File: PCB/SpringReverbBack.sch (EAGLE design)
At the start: 39 parts, among them IC4_DRV_RCVR TL072

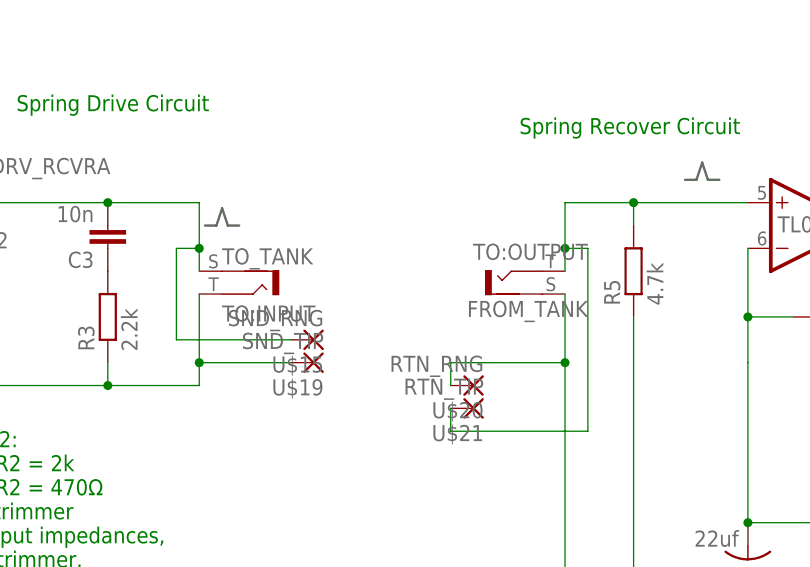
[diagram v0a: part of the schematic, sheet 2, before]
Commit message: Updated to Eagle 7.2
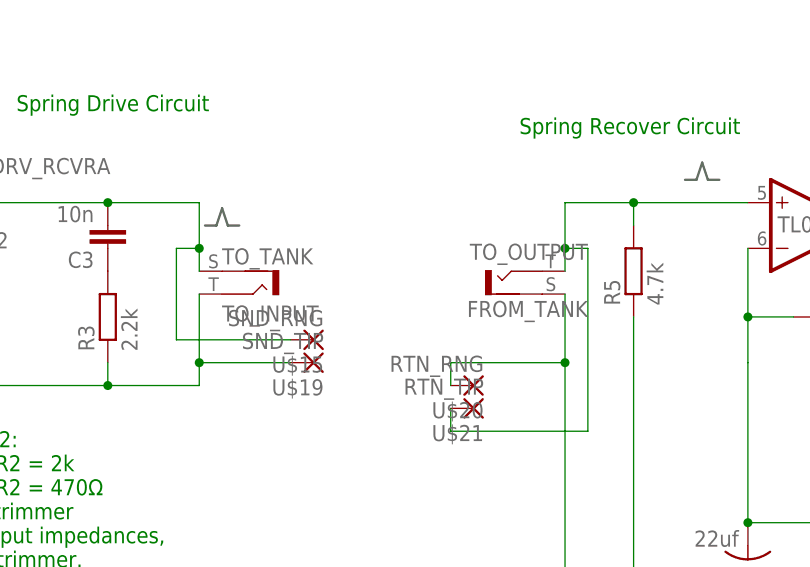
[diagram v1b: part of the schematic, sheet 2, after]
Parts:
- renumbered TO:INPUT to TO_INPUT, TO:OUTPUT to TO_OUTPUT
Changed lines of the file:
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@@
 <?xml version="1.0" encoding="utf-8"?>
 <!DOCTYPE eagle SYSTEM "eagle.dtd">
-<eagle version="6.4">
+<eagle version="7.2.0">
 <drawing>
 <settings>
@@
 <part name="C2" library="SparkFun-Passives" deviceset="CAP_POL" device="PTH2" value="10uf"/>
 <part name="SUPPLY4" library="supply2" deviceset="GND" device=""/>
-<part name="TO:INPUT" library="con-lumberg" deviceset="BTOR1" device="" value="TO_TANK"/>
+<part name="TO_INPUT" library="con-lumberg" deviceset="BTOR1" device="" value="TO_TANK"/>
 <part name="R3" library="TomW" deviceset="R-EU_" device="STANDARD_RESISTOR" value="2.2k"/>
 <part name="C3" library="TomW" deviceset="C-EU" device="050-024X044" value="10n"/>
-<part name="TO:OUTPUT" library="con-lumberg" deviceset="BTOR1" device="" value="FROM_TANK"/>
+<part name="TO_OUTPUT" library="con-lumberg" deviceset="BTOR1" device="" value="FROM_TANK"/>
 <part name="R4" library="TomW" deviceset="R-EU_" device="STANDARD_RESISTOR" value="22R"/>
 <part name="C8" library="SparkFun-Passives" deviceset="CAP_POL" device="PTH2" value="22uf"/>
@@
 <instance part="C2" gate="G$1" x="33.02" y="71.12"/>
 <instance part="SUPPLY4" gate="GND" x="38.1" y="43.18"/>
-<instance part="TO:INPUT" gate="G$1" x="81.28" y="88.9" rot="MR180"/>
+<instance part="TO_INPUT" gate="G$1" x="81.28" y="88.9" rot="MR180"/>
 <instance part="R3" gate="G$1" x="68.58" y="86.36" rot="R90"/>
 <instance part="C3" gate="G$1" x="68.58" y="93.98" rot="R180"/>
@@
 <attribute name="VALUE" x="143.002" y="95.758" size="1.778" layer="96"/>
 </instance>
-<instance part="TO:OUTPUT" gate="G$1" x="116.84" y="91.44" smashed="yes" rot="MR0">
+<instance part="TO_OUTPUT" gate="G$1" x="116.84" y="91.44" smashed="yes" rot="MR0">
 <attribute name="NAME" x="121.92" y="92.71" size="1.778" layer="95" rot="MR0"/>
 <attribute name="VALUE" x="121.92" y="86.36" size="1.778" layer="96" rot="MR0"/>
@@
 <pinref part="R5" gate="G$1" pin="1"/>
 <pinref part="R4" gate="G$1" pin="2"/>
-<pinref part="TO:OUTPUT" gate="G$1" pin="2"/>
+<pinref part="TO_OUTPUT" gate="G$1" pin="2"/>
 <wire x1="139.7" y1="43.18" x2="132.08" y2="43.18" width="0.1524" layer="91"/>
 <wire x1="132.08" y1="43.18" x2="127" y2="43.18" width="0.1524" layer="91"/>
@@
 <net name="N$4" class="0">
 <segment>
-<pinref part="TO:INPUT" gate="G$1" pin="2"/>
+<pinref part="TO_INPUT" gate="G$1" pin="2"/>
 <wire x1="78.74" y1="99.06" x2="78.74" y2="93.98" width="0.1524" layer="91"/>
 <wire x1="78.74" y1="93.98" x2="78.74" y2="91.44" width="0.1524" layer="91"/>
@@
 <net name="N$7" class="0">
 <segment>
-<pinref part="TO:OUTPUT" gate="G$1" pin="1"/>
+<pinref part="TO_OUTPUT" gate="G$1" pin="1"/>
 <wire x1="119.38" y1="91.44" x2="119.38" y2="93.98" width="0.1524" layer="91"/>
 <wire x1="119.38" y1="93.98" x2="119.38" y2="99.06" width="0.1524" layer="91"/>
@@
 <net name="N$5" class="0">
 <segment>
-<pinref part="TO:INPUT" gate="G$1" pin="1"/>
+<pinref part="TO_INPUT" gate="G$1" pin="1"/>
 <wire x1="78.74" y1="88.9" x2="78.74" y2="81.28" width="0.1524" layer="91"/>
 <wire x1="78.74" y1="81.28" x2="78.74" y2="78.74" width="0.1524" layer="91"/>
